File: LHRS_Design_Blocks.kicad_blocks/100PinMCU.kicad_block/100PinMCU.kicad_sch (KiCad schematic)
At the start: 12 parts, among them U1 LMR51635XDDCR

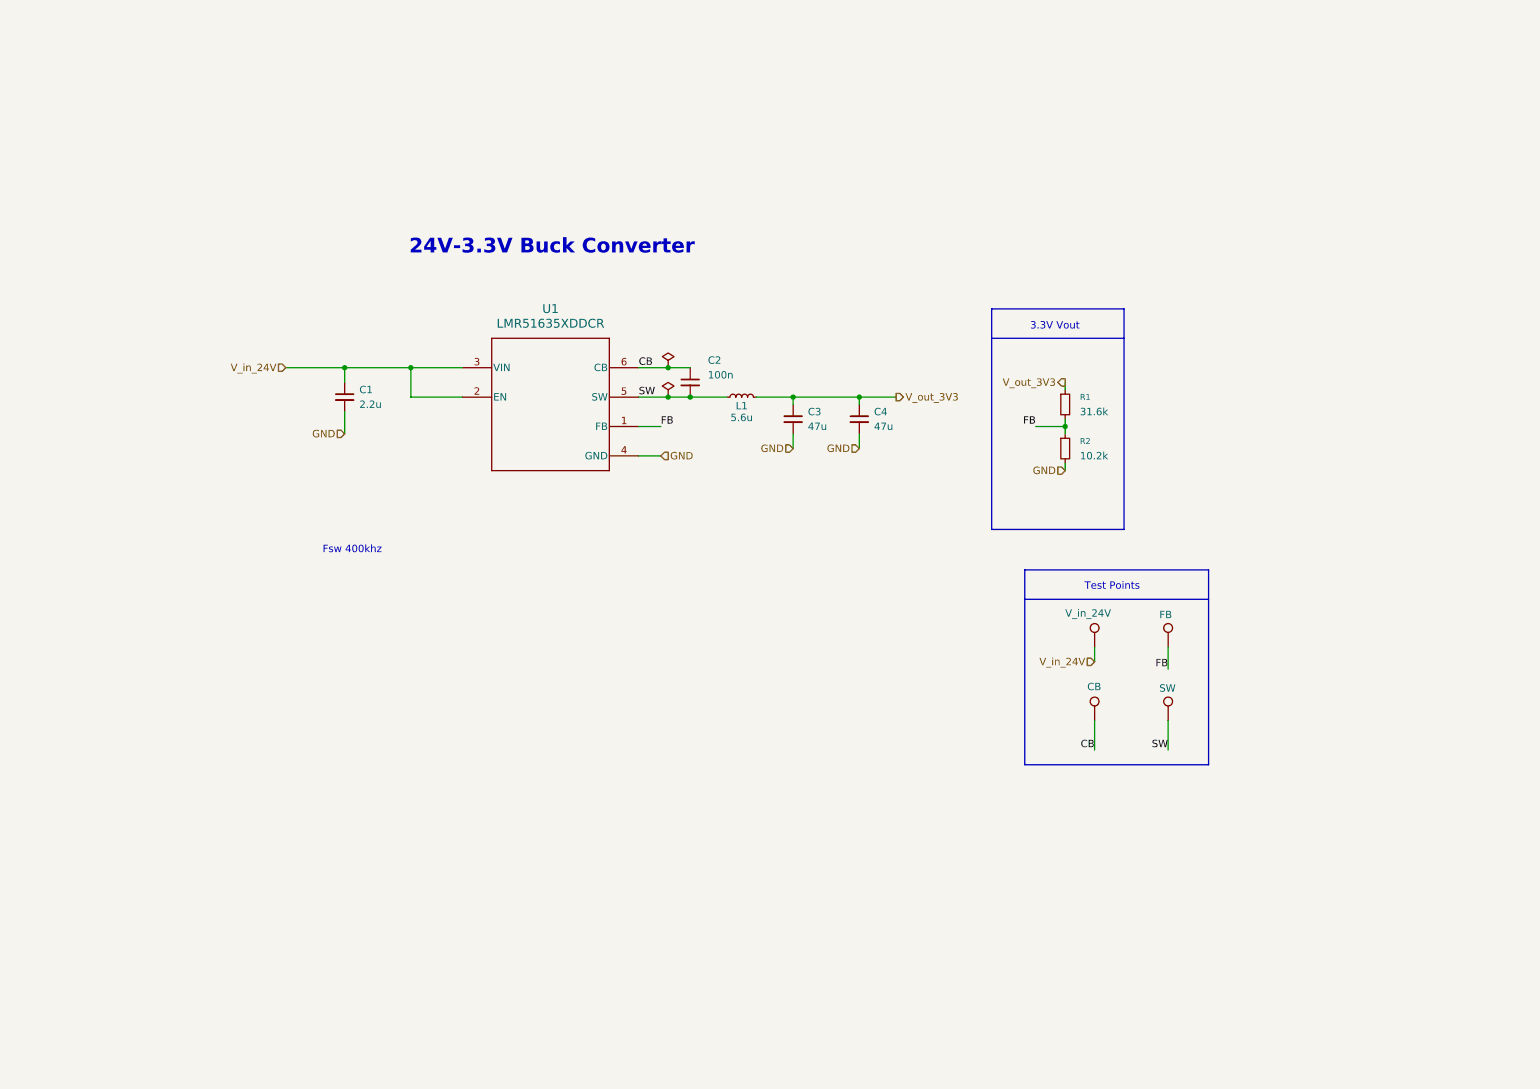
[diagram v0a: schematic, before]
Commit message: UTSVT to LHRS
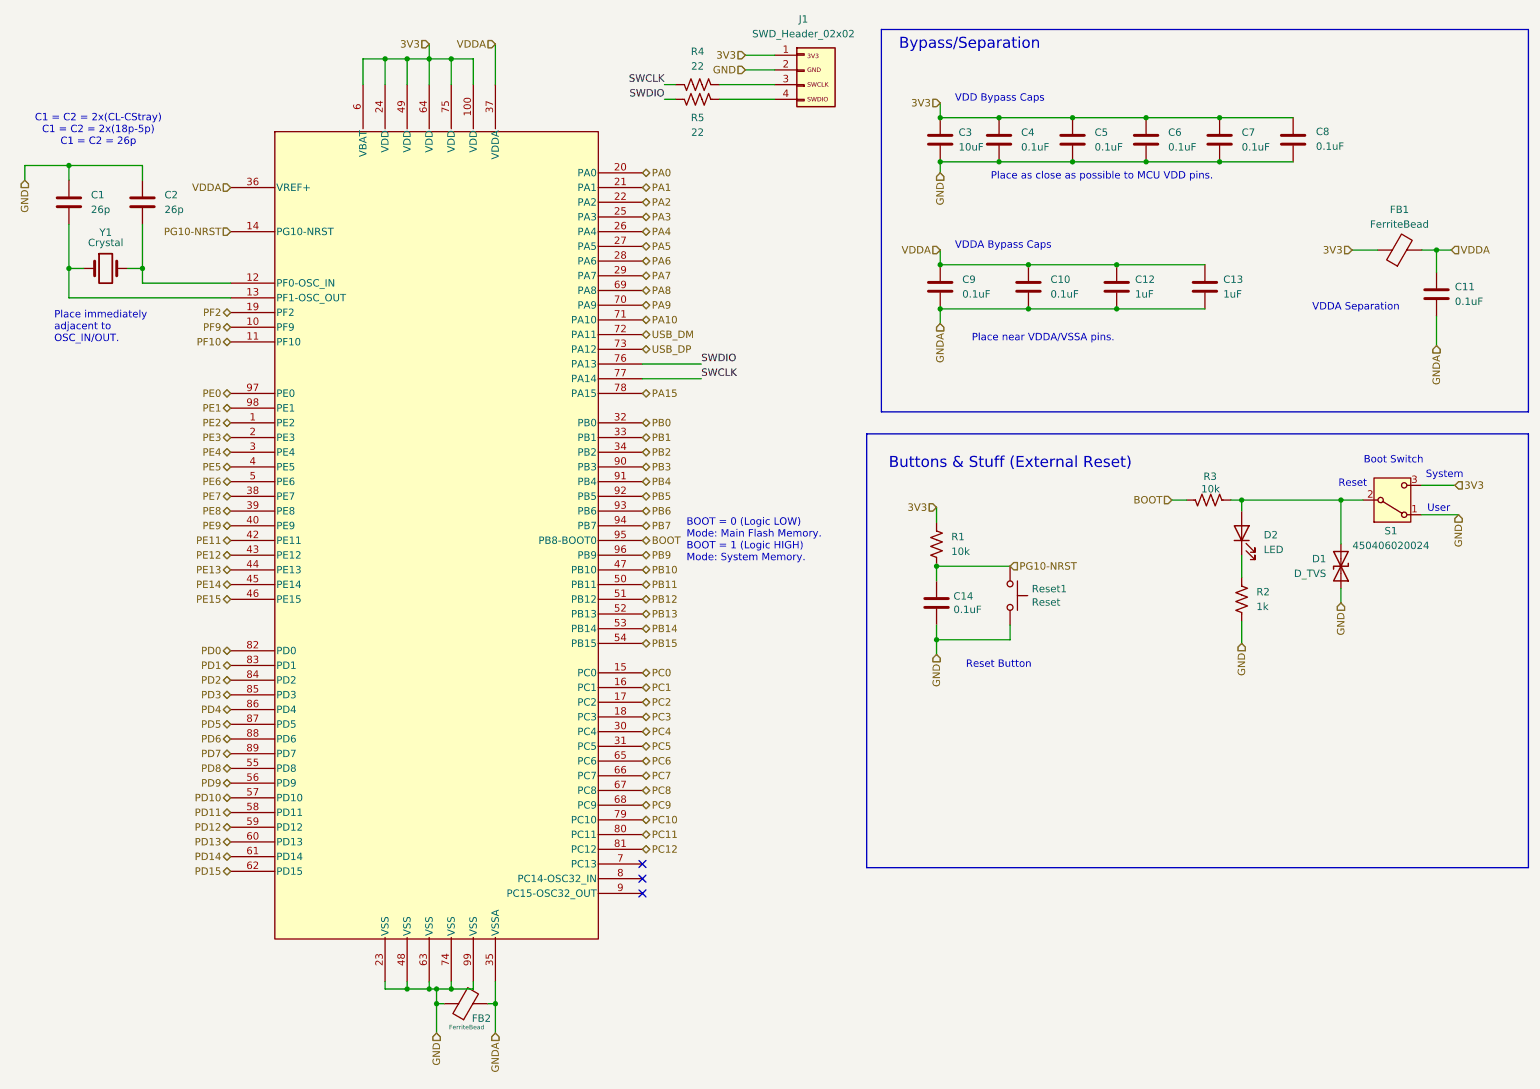
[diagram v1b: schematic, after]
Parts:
- removed C1: 2.2u, Capacitor_SMD:C_0805_2012Metric_Pad1.18x1.45mm_HandSolder, symbol Device:C_Small
- removed C2: 100n, Resistor_SMD:R_0201_0603Metric_Pad0.64x0.40mm_HandSolder, symbol Device:C_Small
- removed C3, C4: 47u, Capacitor_SMD:C_1210_3225Metric_Pad1.33x2.70mm_HandSolder, symbol Device:C_Small
- removed L1: 5.6u, Inductor_SMD:L_TDK_SLF6025, symbol Device:L_Small
- removed R1: 31.6k, Resistor_SMD:R_0603_1608Metric, symbol Device:R_Small
- removed R2: 10.2k, Resistor_SMD:R_0603_1608Metric, symbol Device:R_Small
- removed TP?: FB, TestPoint:TestPoint_THTPad_D3.0mm_Drill1.5mm, symbol Connector:TestPoint
- removed TP?: SW, TestPoint:TestPoint_THTPad_D3.0mm_Drill1.5mm, symbol Connector:TestPoint
- removed TP?: CB, TestPoint:TestPoint_THTPad_D3.0mm_Drill1.5mm, symbol Connector:TestPoint
- removed TP?: V_in_24V, TestPoint:TestPoint_THTPad_D3.0mm_Drill1.5mm, symbol Connector:TestPoint
- removed U1: LMR51635XDDCR, UTSVT_ICs:DDC0006A-MFG, symbol 2026-04-25_18-34-12:LMR51635XDDCR
- added C1, C2: 26p, Capacitor_SMD:C_0603_1608Metric_Pad1.08x0.95mm_HandSolder, symbol Device:C
- added C10, C11, C14, C4, C5, C6, C7, C8, C9: 0.1uF, Capacitor_SMD:C_0603_1608Metric_Pad1.08x0.95mm_HandSolder, symbol Device:C
- added C12, C13: 1uF, Capacitor_SMD:C_0603_1608Metric_Pad1.08x0.95mm_HandSolder, symbol Device:C
- added C3: 10uF, Capacitor_SMD:C_0805_2012Metric, symbol Device:C
- added D1: D_TVS, Diode_SMD:D_SOD-323, symbol Device:D_TVS
- added D2: LED, LED_SMD:LED_0201_0603Metric, symbol Device:LED
- added FB1, FB2: FerriteBead, Capacitor_SMD:C_0603_1608Metric_Pad1.08x0.95mm_HandSolder, symbol Device:FerriteBead
- added J1: SWD_Header_02x02, LHRS_Connectors:SWD_Conn, symbol 100PinMCU:SWD_Header_02x02
- added R1, R3: 10k, Resistor_SMD:R_0603_1608Metric_Pad0.98x0.95mm_HandSolder, symbol Device:R_US
- added R2: 1k, Resistor_SMD:R_0603_1608Metric_Pad0.98x0.95mm_HandSolder, symbol Device:R_US
- added R4, R5: 22, Resistor_SMD:R_0603_1608Metric_Pad0.98x0.95mm_HandSolder, symbol Device:R_US
- added Reset1: Reset, LHRS_Special:TL3365AF180QG, symbol Switch:SW_Push
- added S1: 450406020024, LHRS_Special:BootSW, symbol Switch:SW_SPDT
- added U2: STM32G491VET6_1, LHRS_ICs:LQFP_491VET6_STM, symbol lhrs_ics:STM32G491VET6_1
- added Y1: Crystal, LHRS_Passives:Crystal_SMD_Abracon_ABM3-2Pin_5.0x3.2mm, symbol Device:Crystal
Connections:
- net GND: now also C1.1, C14.2, C2.1, C3.2, C4.2, C5.2, C6.2, C7.2, C8.2, D1.1 (A1), FB2.1, J1.2 (Pin_2), R2.2, Reset1.2, S1.1 (A), U2.23 (VSS), U2.48 (VSS), U2.63 (VSS), U2.74 (VSS), U2.99 (VSS)
- new net: C1.2, U2.13 (PF1-OSC_OUT), Y1.1
- new net: C2.2, U2.12 (PF0-OSC_IN), Y1.2
- new net: D2.1 (K), R2.1
- new net: J1.3 (Pin_3), R4.2
- new net: J1.4 (Pin_4), R5.2
- new net: D1.2 (A2), D2.2 (A), R3.2, S1.2 (B)
- new net 3V3: C3.1, C4.1, C5.1, C6.1, C7.1, C8.1, FB1.1, J1.1 (Pin_1), R1.2, S1.3 (C), U2.100 (VDD), U2.24 (VDD), U2.49 (VDD), U2.6 (VBAT), U2.64 (VDD), U2.75 (VDD)
- new net BOOT: R3.1, U2.95 (PB8-BOOT0)
- new net GNDA: C10.2, C11.2, C12.2, C13.2, C9.2, FB2.2, U2.35 (VSSA)
- new net PA0: U2.20 (PA0)
- new net PA1: U2.21 (PA1)
- new net PA10: U2.71 (PA10)
- new net PA15: U2.78 (PA15)
- new net PA2: U2.22 (PA2)
- new net PA3: U2.25 (PA3)
- new net PA4: U2.26 (PA4)
- new net PA5: U2.27 (PA5)
- new net PA6: U2.28 (PA6)
- new net PA7: U2.29 (PA7)
- new net PA8: U2.69 (PA8)
- new net PA9: U2.70 (PA9)
- new net PB0: U2.32 (PB0)
- new net PB1: U2.33 (PB1)
- new net PB10: U2.47 (PB10)
- new net PB11: U2.50 (PB11)
- new net PB12: U2.51 (PB12)
- new net PB13: U2.52 (PB13)
- new net PB14: U2.53 (PB14)
- new net PB15: U2.54 (PB15)
- new net PB2: U2.34 (PB2)
- new net PB3: U2.90 (PB3)
- new net PB4: U2.91 (PB4)
- new net PB5: U2.92 (PB5)
- new net PB6: U2.93 (PB6)
- new net PB7: U2.94 (PB7)
- new net PB9: U2.96 (PB9)
- new net PC0: U2.15 (PC0)
- new net PC1: U2.16 (PC1)
- new net PC10: U2.79 (PC10)
- new net PC11: U2.80 (PC11)
- new net PC12: U2.81 (PC12)
- new net PC2: U2.17 (PC2)
- new net PC3: U2.18 (PC3)
- new net PC4: U2.30 (PC4)
- new net PC5: U2.31 (PC5)
- new net PC6: U2.65 (PC6)
- new net PC7: U2.66 (PC7)
- new net PC8: U2.67 (PC8)
- new net PC9: U2.68 (PC9)
- new net PD0: U2.82 (PD0)
- new net PD1: U2.83 (PD1)
- new net PD10: U2.57 (PD10)
- new net PD11: U2.58 (PD11)
- new net PD12: U2.59 (PD12)
- new net PD13: U2.60 (PD13)
- new net PD14: U2.61 (PD14)
- new net PD15: U2.62 (PD15)
- new net PD2: U2.84 (PD2)
- new net PD3: U2.85 (PD3)
- new net PD4: U2.86 (PD4)
- new net PD5: U2.87 (PD5)
- new net PD6: U2.88 (PD6)
- new net PD7: U2.89 (PD7)
- new net PD8: U2.55 (PD8)
- new net PD9: U2.56 (PD9)
- new net PE0: U2.97 (PE0)
- new net PE1: U2.98 (PE1)
- new net PE11: U2.42 (PE11)
- new net PE12: U2.43 (PE12)
- new net PE13: U2.44 (PE13)
- new net PE14: U2.45 (PE14)
- new net PE15: U2.46 (PE15)
- new net PE2: U2.1 (PE2)
- new net PE3: U2.2 (PE3)
- new net PE4: U2.3 (PE4)
- new net PE5: U2.4 (PE5)
- new net PE6: U2.5 (PE6)
- new net PE7: U2.38 (PE7)
- new net PE8: U2.39 (PE8)
- new net PE9: U2.40 (PE9)
- new net PF10: U2.11 (PF10)
- new net PF2: U2.19 (PF2)
- new net PF9: U2.10 (PF9)
- new net PG10-NRST: C14.1, R1.1, Reset1.1, U2.14 (PG10-NRST)
- new net SWCLK: R4.1, U2.77 (PA14)
- new net SWDIO: R5.1, U2.76 (PA13)
- new net USB_DM: U2.72 (PA11)
- new net USB_DP: U2.73 (PA12)
- new net VDDA: C10.1, C11.1, C12.1, C13.1, C9.1, FB1.2, U2.36 (VREF+), U2.37 (VDDA)
- no-connect marks 0 -> 3
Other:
- note added: "BOOT = 0 (Logic LOW) Mode: Main Flash Memory. BOOT = 1 (Logic HIGH) Mode: System Memory."
- note added: "Boot Switch"
- note added: "Buttons & Stuff (External Reset)"
- note added: "Bypass/Separation"
- note added: "C1 = C2 = 2x(CL-CStray) C1 = C2 = 2x(18p-5p) C1 = C2 = 26p"
- note added: "Place as close as possible to MCU VDD pins."
- note added: "Place immediately adjacent to OSC_IN/OUT."
- note added: "Place near VDDA/VSSA pins."
- note added: "Reset"
- note added: "Reset Button"
- note added: "System"
- note added: "User"
- note added: "VDD Bypass Caps"
- note added: "VDDA Bypass Caps"
- note added: "VDDA Separation"
- note removed: "24V-3.3V Buck Converter"
- note removed: "3.3V Vout"
- note removed: "Fsw 400khz"
- note removed: "Test Points"
